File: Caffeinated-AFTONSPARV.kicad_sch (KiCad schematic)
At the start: 33 parts, among them J1 Conn_01x02, J2 Conn_01x04, J3 TagConnect, Q1 AO3400A, Q2 AO3400A, Q3 AO3400A, SW1 SW_Push, U1 ESP32-C3-MINI-1, U2 SY8201ABC

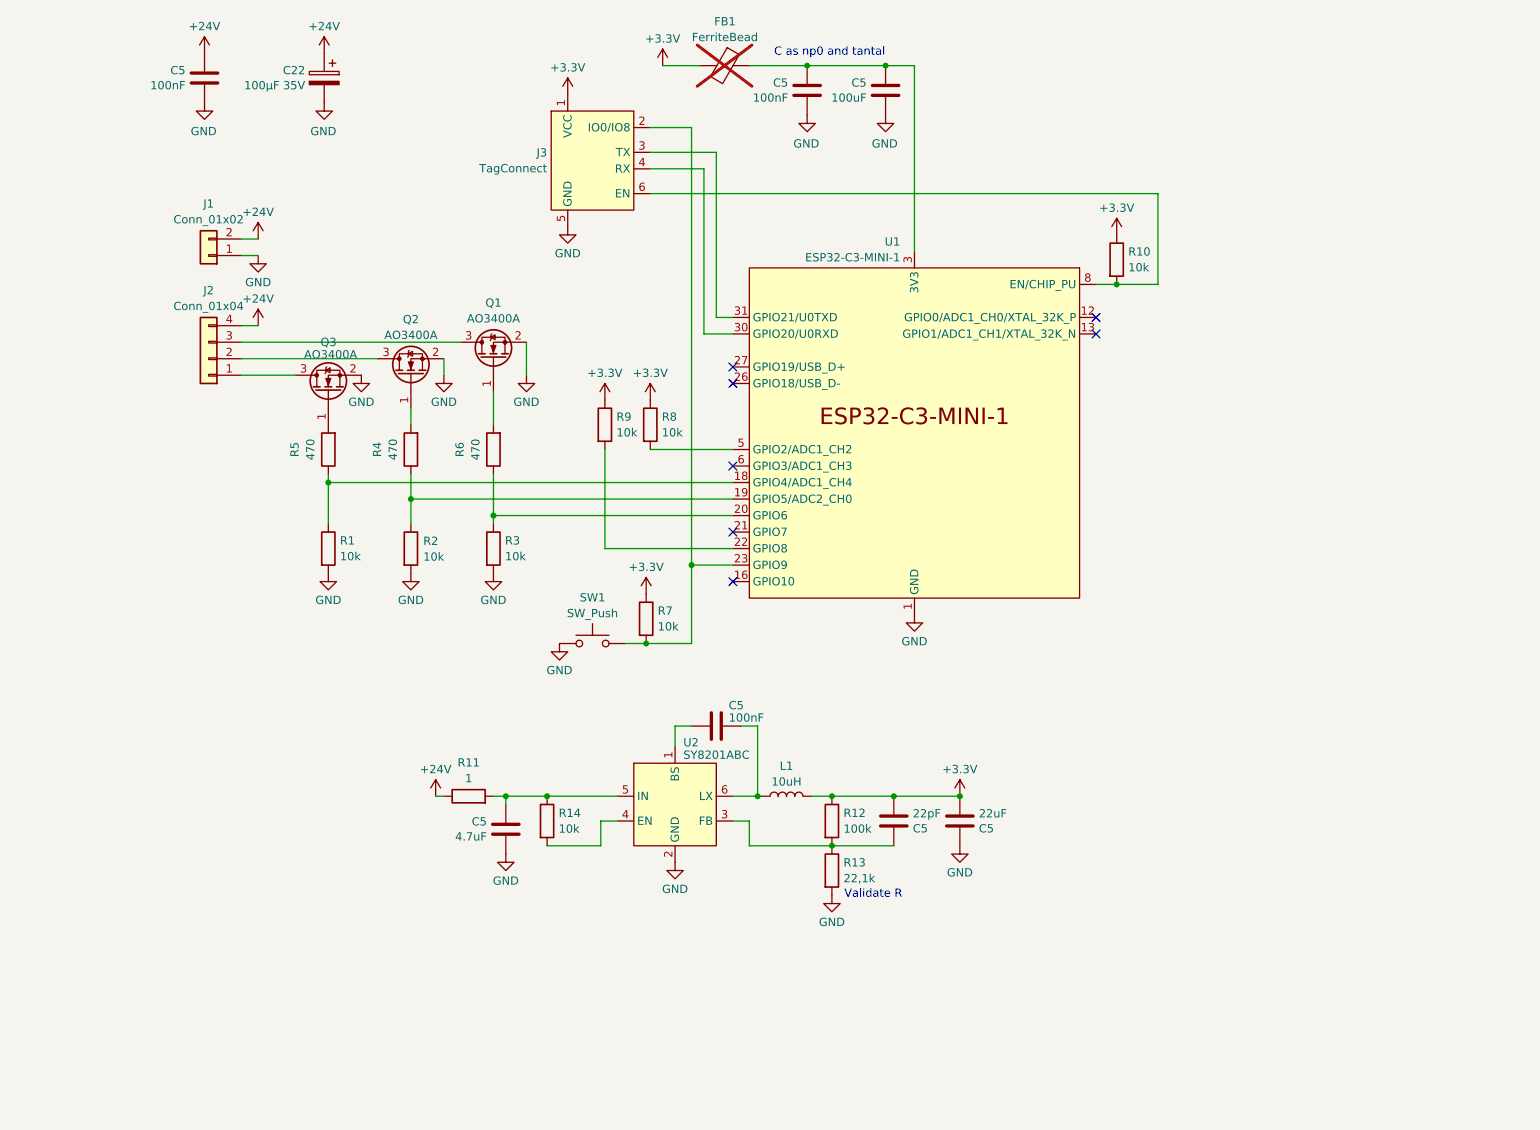
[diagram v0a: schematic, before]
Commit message: feat(): Rework and finalize design
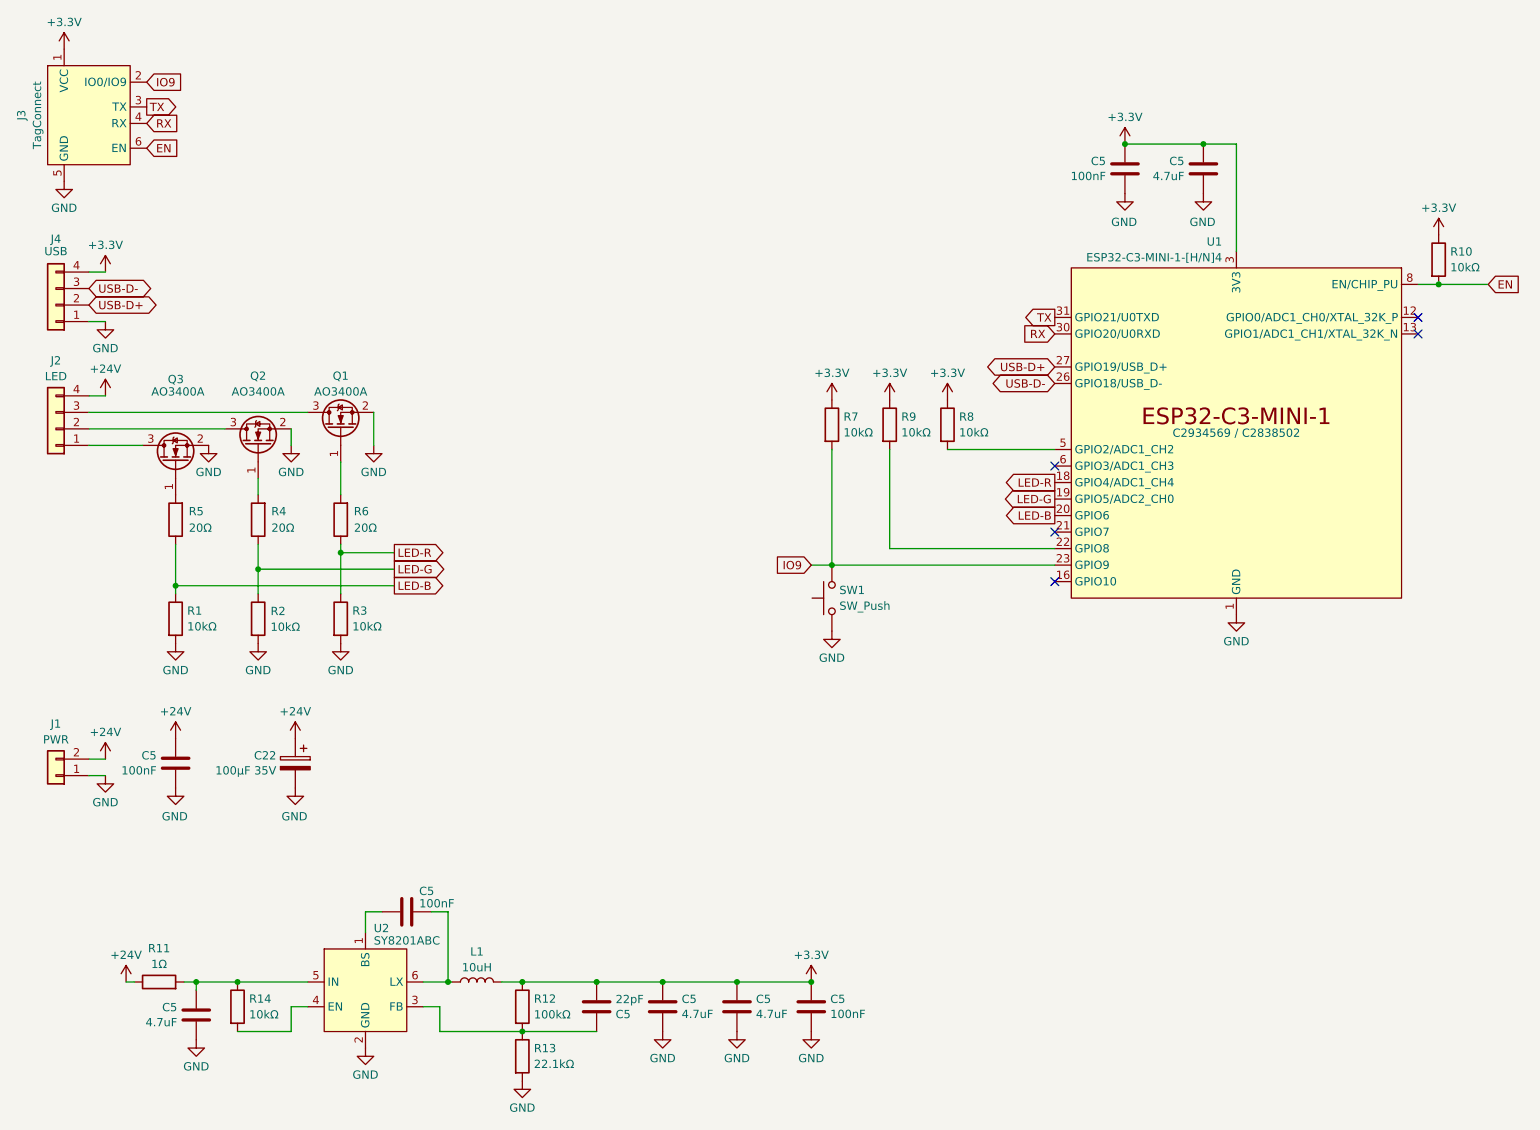
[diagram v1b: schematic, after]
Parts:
- removed C5: 100uF, Capacitor_SMD:C_0603_1608Metric, symbol Device:C
- removed C5: 22uF, Capacitor_SMD:C_0603_1608Metric, symbol Device:C
- removed FB1: FerriteBead, PCM_Ferrite_SMD_AKL:Ferrite_0603_1608Metric, symbol Device:FerriteBead
- added C5: 100nF, Capacitor_SMD:C_0603_1608Metric, symbol Device:C
- added C5 (x3): 4.7uF, Capacitor_SMD:C_0805_2012Metric, symbol Device:C
- added J4: USB, Connector_PinSocket_1.00mm:PinSocket_1x04_P1.00mm_Vertical, symbol Connector_Generic:Conn_01x04
- C22: LCSC C19702 -> (none)
- C5: LCSC C14663 -> (none)
- J1: value Conn_01x02 -> PWR; now left out of the parts list
- J2: value Conn_01x04 -> LED; now left out of the parts list
- J3: now left out of the parts list
- Q1, Q2, Q3: LCSC (none) -> C347475
- R1, R10, R14, R2, R3, R7, R8, R9: value 10k -> 10kΩ
- R11: value 1 -> 1Ω
- R12: value 100k -> 100kΩ
- R13: value 22,1k -> 22.1kΩ
- R4, R5, R6: value 470 -> 20Ω
- SW1: footprint Button_Switch_SMD:SW_Push_1P1T_XKB_TS-1187A -> caffeinated-labs:YTS-C005; LCSC (none) -> C318884
- U1: value ESP32-C3-MINI-1 -> ESP32-C3-MINI-1-[H/N]4; LCSC (none) -> C2934569 / C2838502
- U2: LCSC (none) -> C108052
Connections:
- net +3.3V: now also C5.1, U1.3 (3V3), C5.1, C5.1, C5.1, C5.1, J4.4 (Pin_4)
- net GND: now also C5.2, C5.2, C5.2, C5.2, J4.1 (Pin_1)
- net IO9: now reaches J3.2 (IO0/IO9), R7.2, SW1.2, U1.23 (GPIO9)
- net LED-B: now reaches R1.1, R5.1
- net LED-B: now also U1.20 (GPIO6); no longer U1.18 (GPIO4/ADC1_CH4)
- net LED-G: now reaches R2.1, R4.1, U1.19 (GPIO5/ADC2_CH0)
- net LED-R: now reaches R3.1, R6.1
- net LED-R: now also U1.18 (GPIO4/ADC1_CH4); no longer U1.20 (GPIO6)
- net USB-D-: now reaches U1.26 (GPIO18/USB_D-)
- net USB-D-: now also J4.3 (Pin_3)
- net USB-D+: now reaches U1.27 (GPIO19/USB_D+)
- net USB-D+: now also J4.2 (Pin_2)
- net RX: now reaches J3.4 (RX), U1.30 (GPIO20/U0RXD)
- net TX: now reaches J3.3 (TX), U1.31 (GPIO21/U0TXD)
- net EN: now reaches J3.6 (EN), R10.2, U1.8 (EN/CHIP_PU)
- no-connect marks 7 -> 5
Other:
- note removed: "C as np0 and tantal"
- note removed: "Validate R"
- moved on the sheet: C22, C5, J1, J2, J3, L1, Q1, Q2, Q3, R1, R10, R11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
